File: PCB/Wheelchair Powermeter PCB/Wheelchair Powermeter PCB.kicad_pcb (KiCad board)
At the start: 2 copper layers, 76.8 x 63.5 mm, 37 parts, among them J1 USB4085-GF-A_REVB, U1 ESP32-V2, U2 TE4525, U3 4554_IMU_9DOF, U4 MPL3115A2

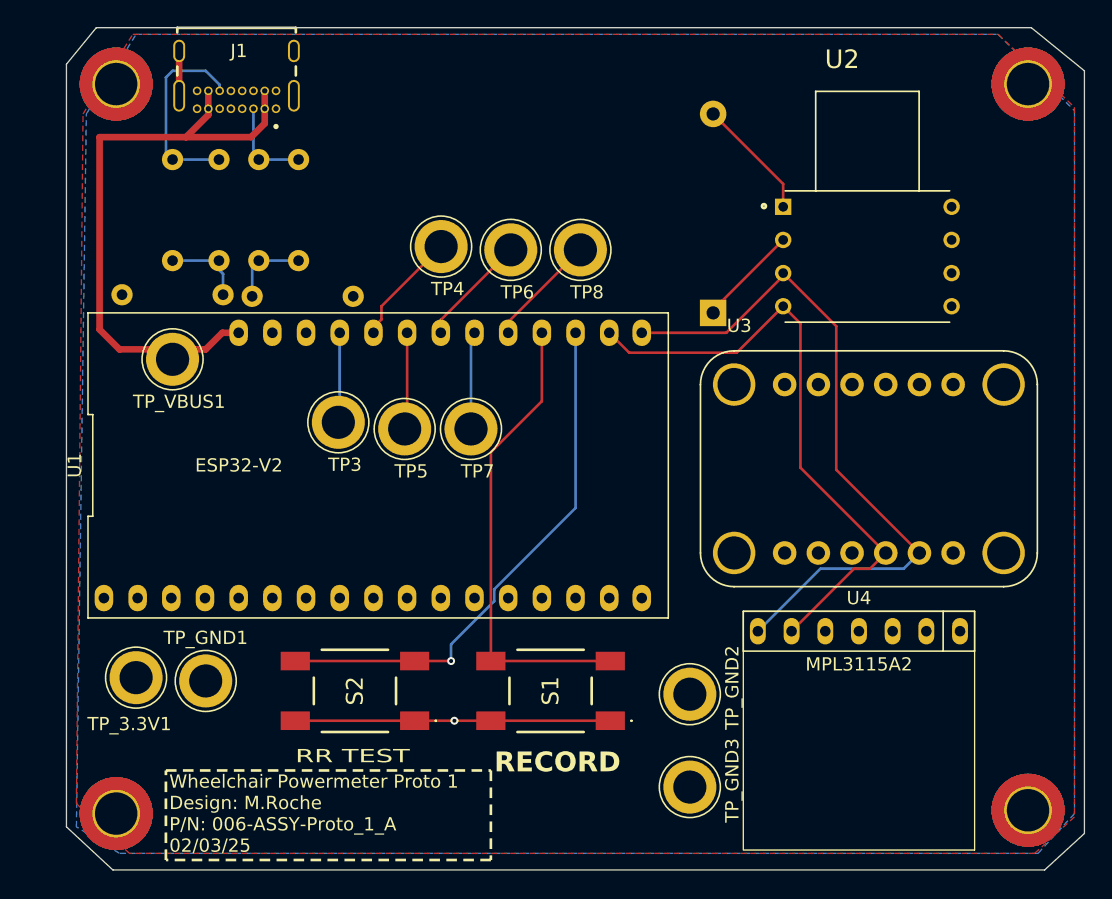
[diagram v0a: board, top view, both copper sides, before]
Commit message: Moooorrrrrrr
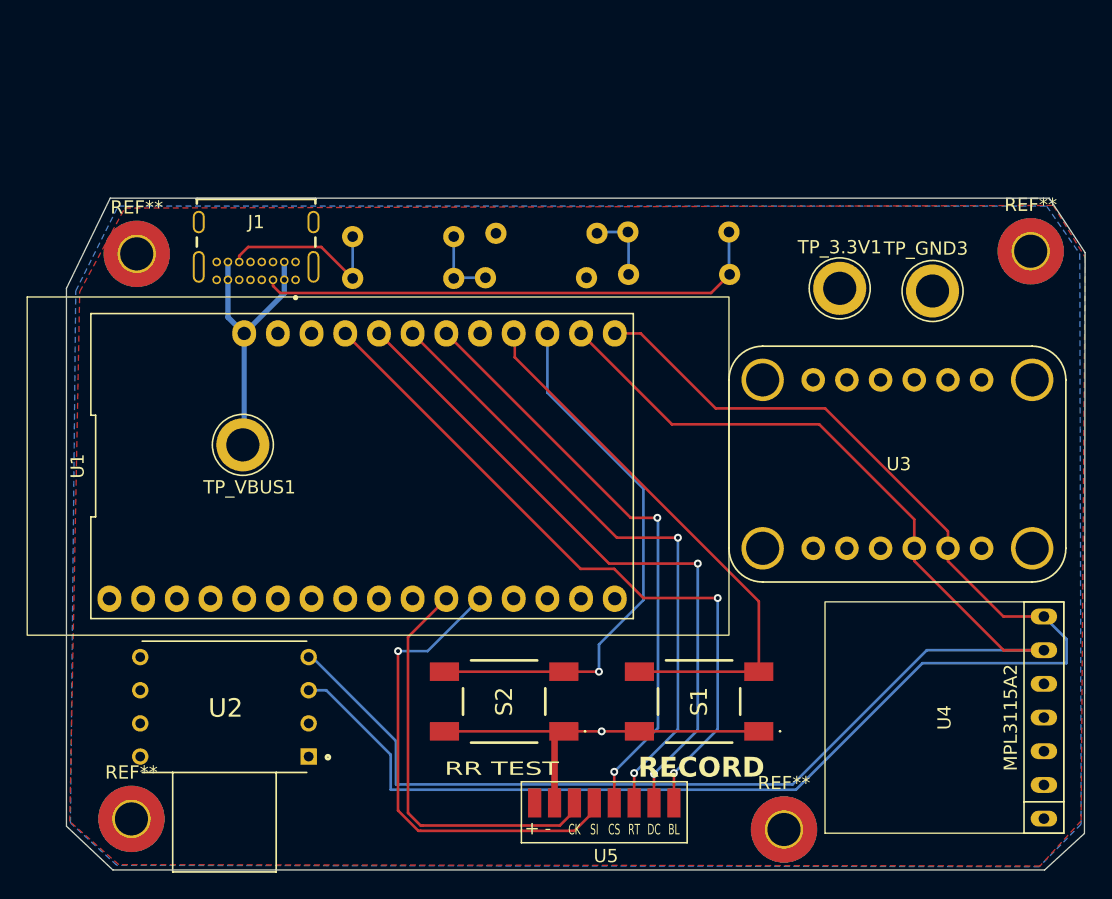
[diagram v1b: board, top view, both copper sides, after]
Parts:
- removed ? (x8): , 
- removed C1: C, Capacitor_THT:CP_Axial_L10.0mm_D4.5mm_P15.00mm_Horizontal
- removed REF1, REF2, REF3, REF4: MountingHole_3.2mm_M3_ISO14580_Pad_TopBottom, MountingHole:MountingHole_3.2mm_M3_ISO14580_Pad_TopBottom
- removed TP3, TP4, TP5, TP6, TP7, TP8, TP_GND1, TP_GND2: TestPoint, TestPoint:TestPoint_Loop_D3.80mm_Drill2.5mm
- added REF**: MountingHole_2.5mm_Pad_TopBottom, MountingHole:MountingHole_2.5mm_Pad_TopBottom, F.Cu at (78.4, 119.4)
- added REF**: MountingHole_2.5mm_Pad_TopBottom, MountingHole:MountingHole_2.5mm_Pad_TopBottom, F.Cu at (146.2, 76.6)
- added REF**: MountingHole_2.5mm_Pad_TopBottom, MountingHole:MountingHole_2.5mm_Pad_TopBottom, F.Cu at (127.6, 120.2)
- added REF**: MountingHole_2.5mm_Pad_TopBottom, MountingHole:MountingHole_2.5mm_Pad_TopBottom, F.Cu at (78.8, 76.8)
- added U5: ~, Adafruit:SPI_Screen, F.Cu at (114.0, 118.2)
- R5, R6: value 100KR -> 100R
- U1: value ESP32-V2 -> ESP32-S3; footprint Adafruit:ESP32 V3 -> Adafruit:ESP32-S3
- moved TP_3.3V1 60.6 mm to (131.8, 79.4)
- moved U2 59.2 mm to (85.4, 111.0), turned to 180 degrees
- moved TP_GND3 41.6 mm to (138.8, 79.6), turned to 180 degrees
- moved R2 35.9 mm to (123.5, 75.2), turned to 180 degrees
- moved R3 33.6 mm to (123.5, 78.3), turned to 180 degrees
- moved R6 26.4 mm to (113.5, 75.2), turned to 180 degrees
- moved U1 22.2 mm to (73.2, 92.6)
- moved R5 19.8 mm to (105.1, 78.6), turned to 0 degrees
- moved R4 16.3 mm to (95.1, 78.7), turned to 0 degrees
- moved U4 15.4 mm to (147.2, 111.8), turned to 90 degrees
- moved J1 13.0 mm to (87.8, 74.4)
- moved R1 11.6 mm to (95.1, 75.5), turned to 0 degrees
- moved S2 11.3 mm to (106.5, 110.5)
- moved S1 11.2 mm to (121.2, 110.5)
- moved TP_VBUS1 8.35 mm to (86.8, 91.2)
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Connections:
- J1 pad A4: Net-(U1-VBAT) -> /POWER
- J1 pad A9: Net-(U1-VBAT) -> /POWER
- J1 pad B4: Net-(U1-VBAT) -> /POWER
- J1 pad B9: Net-(U1-VBAT) -> /POWER
- TP_VBUS1 pad 1: Net-(U1-VBAT) -> /POWER
- U1 pad 11: unconnected-(U1-SCK-Pad11) -> Net-(U1-SCK)
- U1 pad 12: unconnected-(U1-MOSI-Pad12) -> Net-(U1-MOSI)
- U1 pad 16: (no net) -> unconnected-(U1-TXD0-Pad16)
- U1 pad 17: unconnected-(U1-D37-Pad17) -> /POWER
- U1 pad 18: Net-(U1-VBAT) -> unconnected-(U1-EN-Pad18)
- U1 pad 20: unconnected-(U1-VBUS-Pad20) -> Net-(U1-D13)
- U1 pad 24: Net-(U1-D27) -> unconnected-(U1-D9-Pad24)
- U1 pad 25: Net-(U1-D33) -> Net-(S1-NO_1)
- U1 pad 26: Net-(U1-D15) -> Net-(S2-NO_1)
- U1 pad 27: Net-(S1-NO_1) -> SCL_MCU
- U1 pad 28: Net-(S2-NO_1) -> SDA_MCU
- U1 pad 3: unconnected-(U1-Pad3) -> 3.3V
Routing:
- net SCL_MCU: track 46.5 -> 112.2 mm
- net SDA_MCU: track 52.6 -> 112.5 mm
- net Net-(U1-D13): track 0.00 -> 53.2 mm, vias 0 -> 2
- net Net-(U1-VBAT): track 45.6 -> 0.00 mm
- net Net-(U1-D12): track 6.79 -> 50.7 mm, vias 0 -> 2
- net Net-(U1-D11): track 8.61 -> 47.7 mm, vias 0 -> 2
- net Net-(U1-D10): track 7.33 -> 44.6 mm, vias 0 -> 2
- net Net-(U1-MOSI): track 0.00 -> 36.5 mm, vias 0 -> 1
- net Net-(J1-CC1): track 7.00 -> 38.9 mm
- net Net-(U1-SCK): track 0.00 -> 31.3 mm
- net /POWER: track 0.00 -> 21.3 mm
- net Net-(U1-D15): track 8.51 -> 0.00 mm
- net Net-(U1-D27): track 8.43 -> 0.00 mm
- net 3.3V: track 7.69 -> 0.00 mm
- net Net-(U1-D33): track 7.36 -> 0.00 mm
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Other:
- board size 76.8 x 63.5 mm -> 76.8 x 50.7 mm
- board text added: "Wheelchair Powermeter Proto 2 Design: M.Roche P/N: 006-ASSY-Proto_2_A 02/03/25"
- board text removed: "Wheelchair Powermeter Proto 1 Design: M.Roche P/N: 006-ASSY-Proto_1_A 02/03/25"
